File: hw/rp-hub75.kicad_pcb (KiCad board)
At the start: 2 copper layers, 45 x 52 mm, 41 parts, among them J1 Display Connector, J2 USB_C_Receptacle_USB2.0_16P, J3 Screw_Terminal_01x02, J4 Conn_01x02, J5 USB_A, J6 Conn_01x10, J7 Conn_01x05, U1 AMS1117-3.3, U2 RP2350_60QFN, U3 ZD25WQ80CTIGT, Y1 TXM12M0004322CBCDO00T

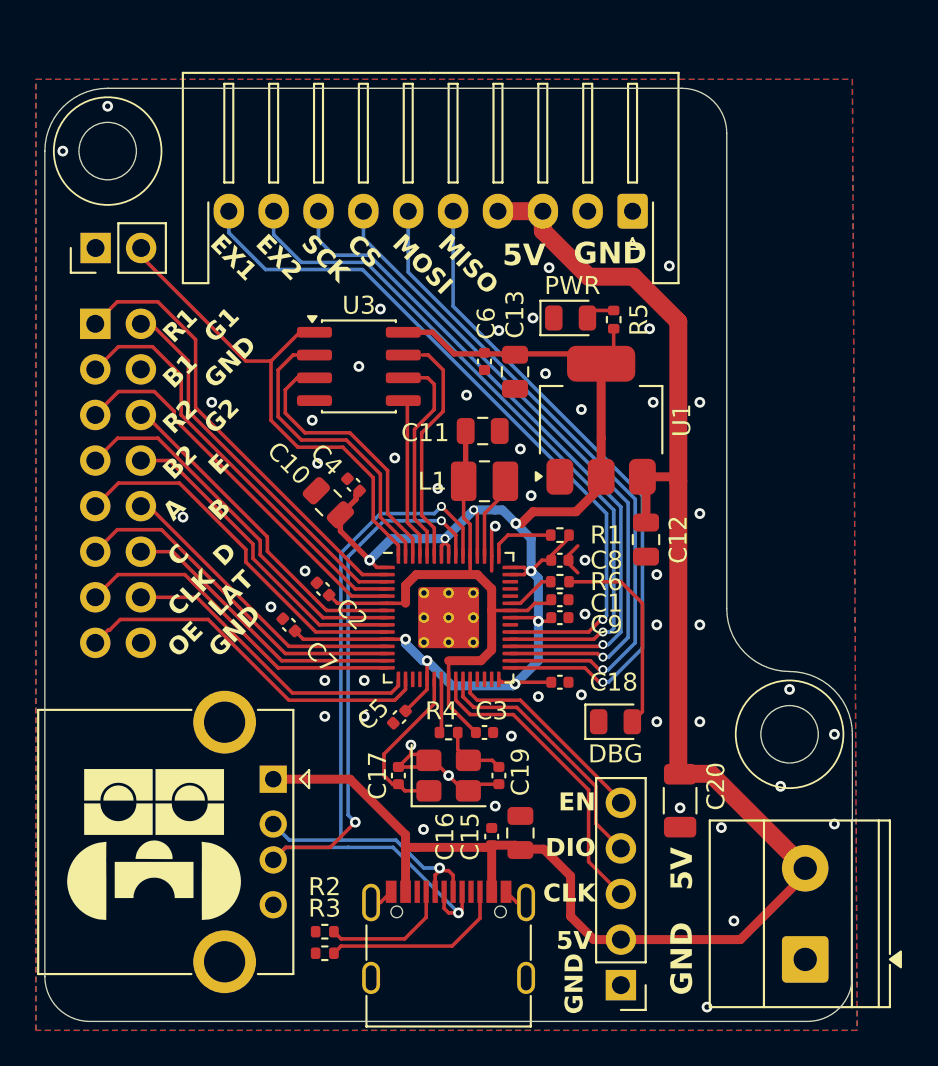
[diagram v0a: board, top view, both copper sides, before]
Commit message: V1.3
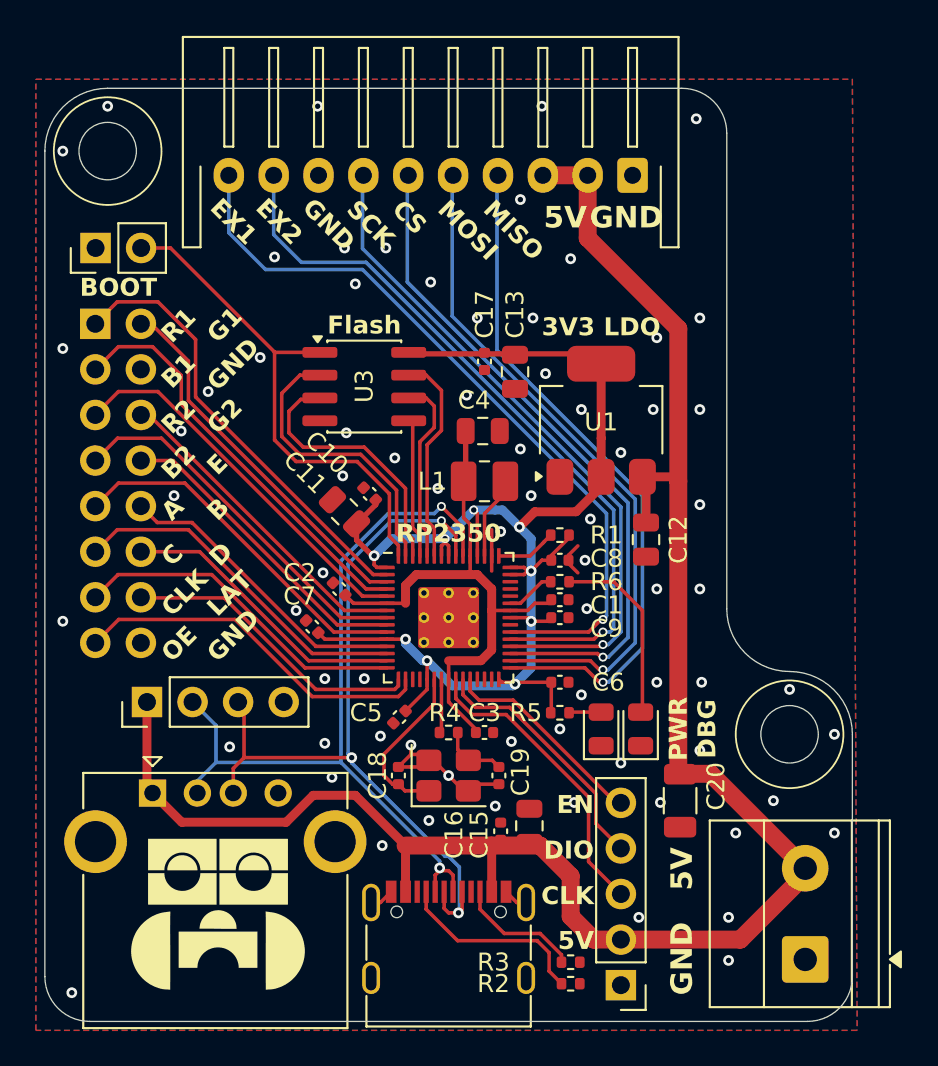
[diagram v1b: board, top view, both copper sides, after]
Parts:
- added J8: Conn_01x04, Connector_PinHeader_2.54mm:PinHeader_1x04_P2.54mm_Vertical, F.Cu at (183.2, 104.7)
- moved D1 23.0 mm to (208.5, 106.2), turned to 90 degrees
- moved R5 22.1 mm to (206.2, 105.3), turned to 0 degrees
- moved R2 14.0 mm to (206.8, 120.4), turned to 0 degrees
- moved R3 13.7 mm to (206.8, 119.2), turned to 0 degrees
- moved J5 6.77 mm to (183.5, 109.8), turned to 0 degrees
- moved J6 2.00 mm to (210.2, 75.3)
- moved D2 1.46 mm to (210.7, 106.2), turned to 90 degrees
- moved C7 1.30 mm to (192.4, 100.5)
- moved U3 1.16 mm to (195.3, 87.1)
- moved C10 1.03 mm to (195.6, 93.1)
- moved C11 1.03 mm to (194.2, 94.1)
- moved C2 0.90 mm to (193.9, 98.4)
- moved C15 0.64 mm to (204.5, 111.6)
- moved C16 0.58 mm to (202.9, 111.9)
- renumbered C4 to C10, C10 to C11, C6 to C17, C17 to C18, C11 to C4, C18 to C6
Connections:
- J6 pad 2: GND -> +5V
- J6 pad 4: +5V -> SPI_MISO
- J6 pad 5: SPI_MISO -> SPI_MOSI
- J6 pad 6: SPI_MOSI -> SPI_CS
- J6 pad 7: SPI_CS -> SPI_SCK
- J6 pad 8: SPI_SCK -> GND
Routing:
- net +5V: track 94.4 -> 106.6 mm
- net D-: track 39.4 -> 45.7 mm
- net Net-(J2-CC1): track 7.23 -> 10.8 mm
- net Net-(J2-CC2): track 10.4 -> 6.98 mm
- net +3V3: track 84.4 -> 81.2 mm
- net SPI_X1: track 39.2 -> 41.2 mm
- net SPI_X2: track 40.2 -> 42.2 mm
- net /QSPI_SCLK: track 12.1 -> 10.5 mm
- net Net-(D2-A): track 11.8 -> 10.4 mm
- net /QSPI_SD0: track 9.01 -> 7.79 mm
- net D+: track 44.0 -> 45.2 mm
- net SPI_MOSI: track 37.1 -> 38.1 mm
- net SPI_CS: track 37.0 -> 38.0 mm
- net SPI_MISO: track 37.2 -> 38.2 mm
- net +1V1: track 32.8 -> 31.9 mm
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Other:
- board text added: "3V3 LDO"
- board text added: "BOOT"
- board text added: "D+"
- board text added: "D-"
- board text added: "Flash"
- board text added: "RP2350"
- board text added: "RP2350 HUB75E"
- board text added: "V1.3"
- board text added: "display driver"
- board text removed: "RP2350 HUB75E driver"
- board text removed: "V1.2"
